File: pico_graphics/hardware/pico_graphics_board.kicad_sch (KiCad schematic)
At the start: 22 parts, among them J1 8bit_thing_bus_connector, J2 HDMI_A, J3 greenpak_i2c, U1 Pico, U2 74LVC245, U3 74LVC245, U4 SLG46826G

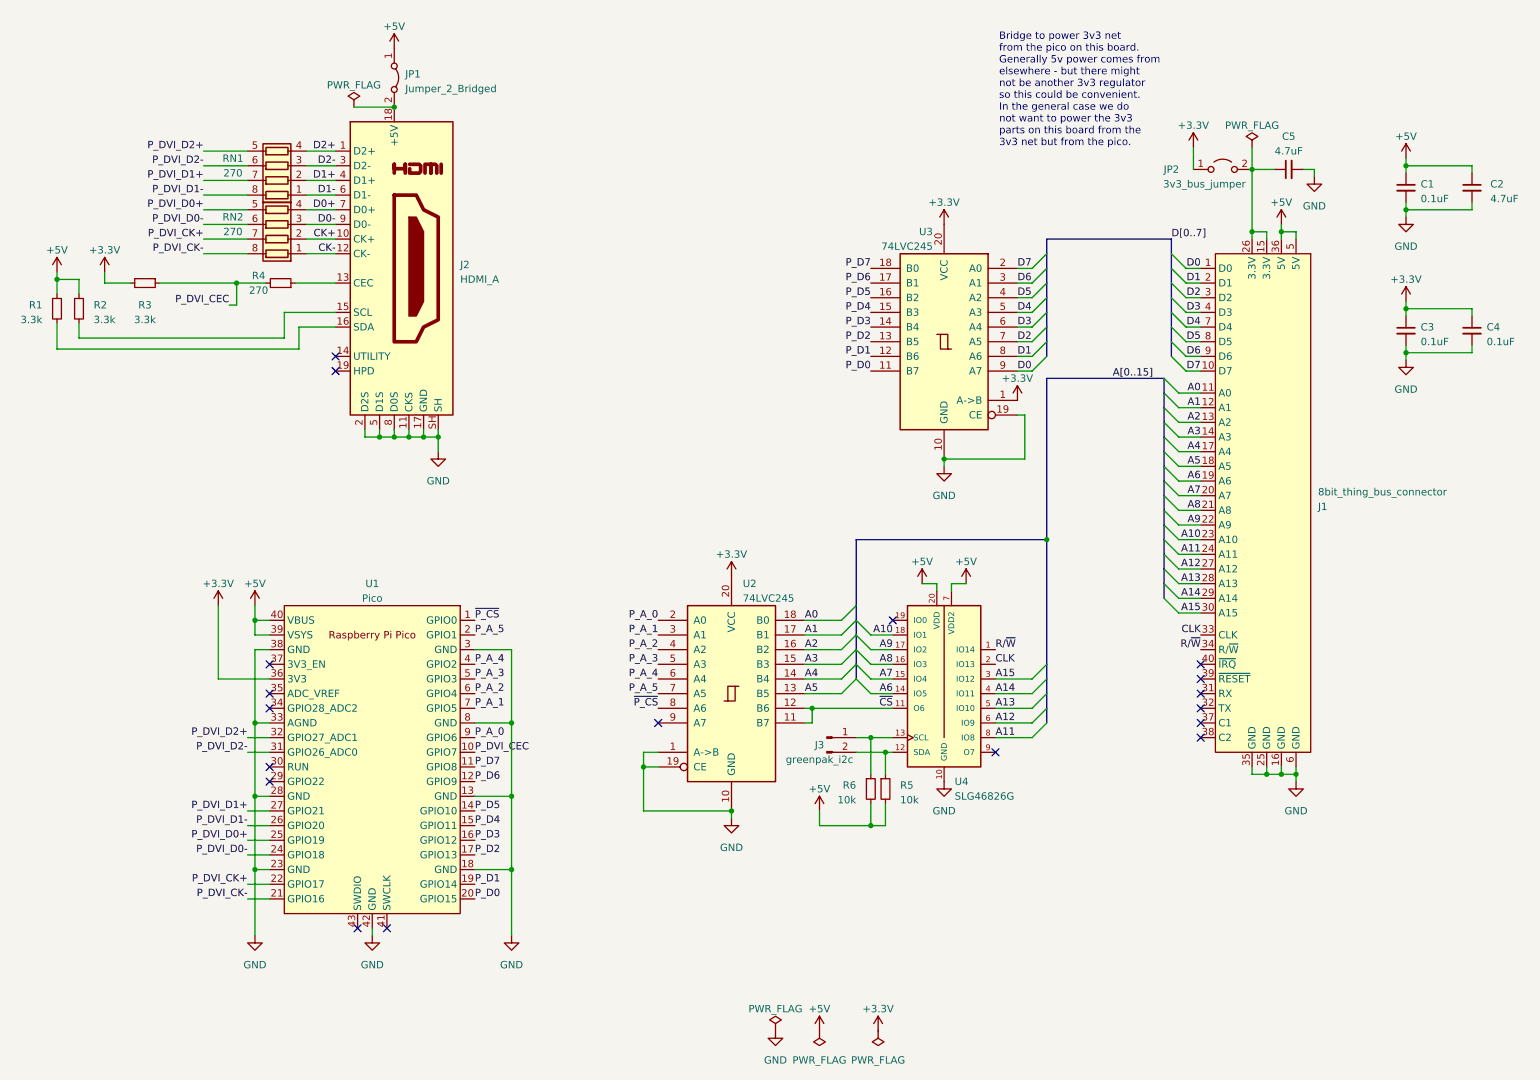
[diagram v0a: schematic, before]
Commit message: Final pico graphics v1.0 board
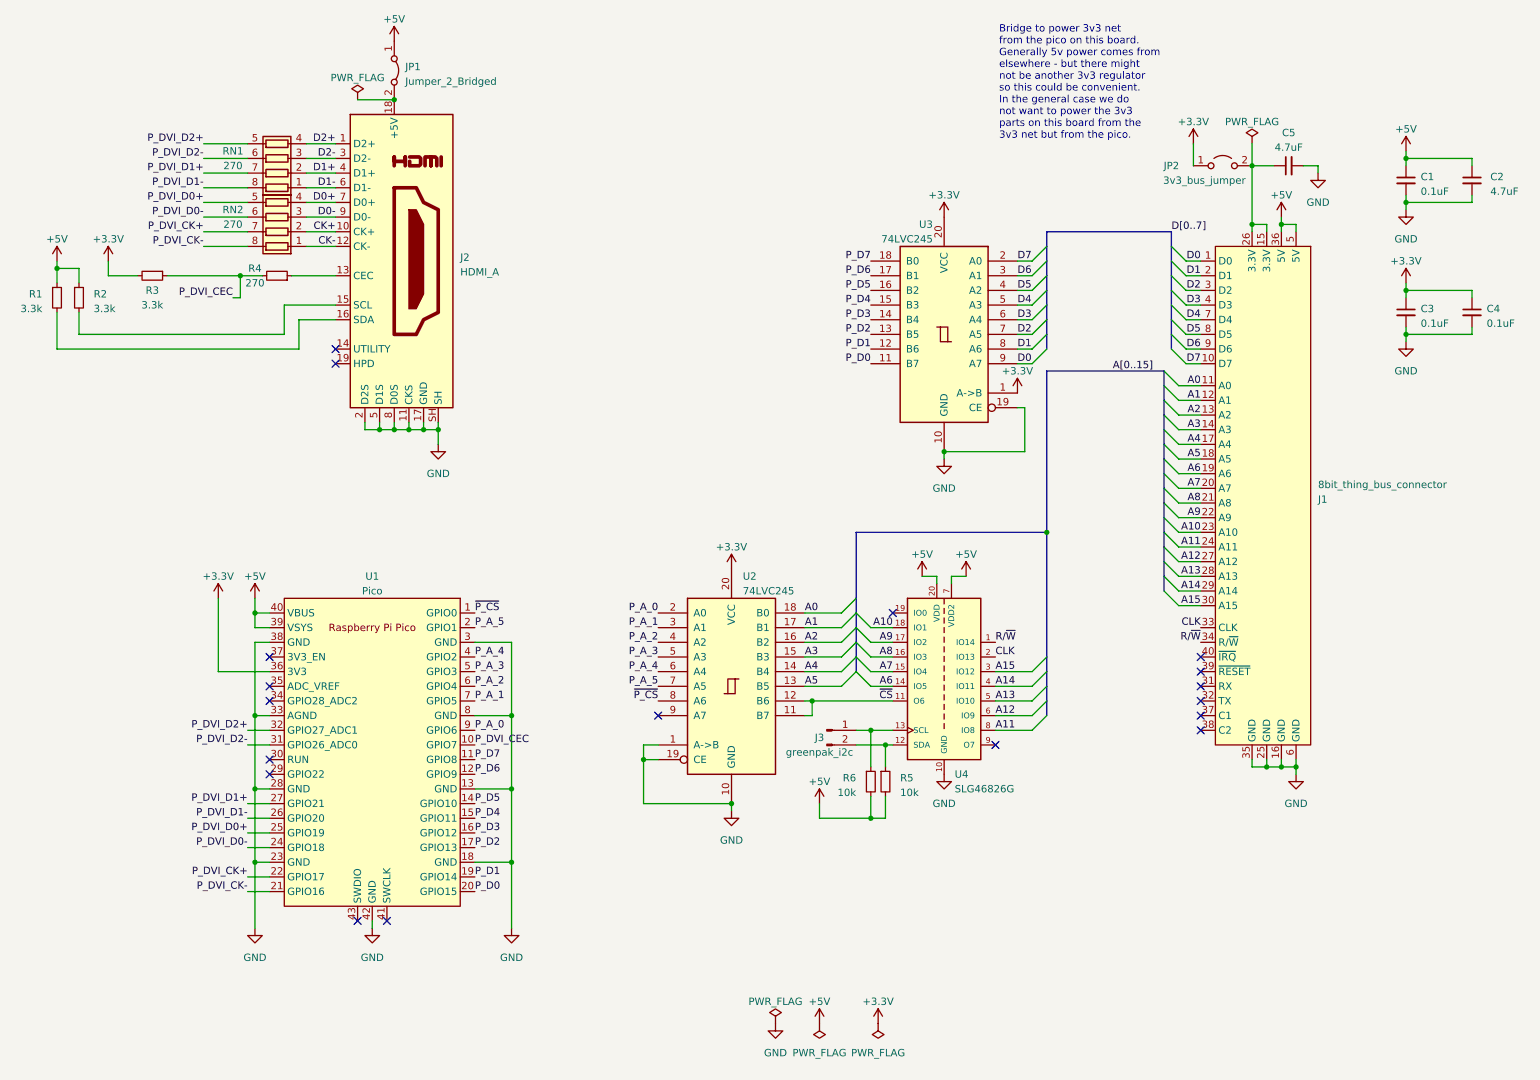
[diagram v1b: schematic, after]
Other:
- moved on the sheet: C1, C2, C3, C4, C5, J1, J2, J3, JP1, JP2, R1, R2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
